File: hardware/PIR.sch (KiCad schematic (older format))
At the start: 3 parts, among them U10 EKMC1601112

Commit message: update
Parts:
- R18, R20: footprint Resistors_SMD:R_0603_HandSoldering -> Resistor_SMD:R_0603_1608Metric_Pad1.05x0.95mm_HandSolder
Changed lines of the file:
@@
 F 0 "R18" V 6050 2275 50  0000 C CNN
 F 1 "R_100k" V 5950 2275 50  0000 C CNN
-F 2 "Resistors_SMD:R_0603_HandSoldering" V 5980 2275 50  0001 C CNN
+F 2 "Resistor_SMD:R_0603_1608Metric_Pad1.05x0.95mm_HandSolder" V 5980 2275 50  0001 C CNN
 F 3 "https://www.digikey.com/product-detail/en/yageo/RC0603JR-07100KL/311-100KGRCT-ND/729645" V 6130 2275 50  0001 C CNN
 F 4 "RC0603JR-07100KL" V 6230 2375 60  0001 C CNN "Part Number"
@@
 F 0 "R20" V 6275 2475 50  0000 C CNN
 F 1 "R_100k" V 6175 2475 50  0000 C CNN
-F 2 "Resistors_SMD:R_0603_HandSoldering" V 6205 2475 50  0001 C CNN
+F 2 "Resistor_SMD:R_0603_1608Metric_Pad1.05x0.95mm_HandSolder" V 6205 2475 50  0001 C CNN
 F 3 "https://www.digikey.com/product-detail/en/yageo/RC0603JR-07100KL/311-100KGRCT-ND/729645" V 6355 2475 50  0001 C CNN
 F 4 "RC0603JR-07100KL" V 6455 2575 60  0001 C CNN "Part Number"

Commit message: order complete
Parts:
- R18, R20: Part Number RC0603JR-07100KL -> ERA-3AEB104V
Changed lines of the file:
@@
 F 2 "Resistor_SMD:R_0603_1608Metric_Pad1.05x0.95mm_HandSolder" V 5980 2275 50  0001 C CNN
 F 3 "https://www.digikey.com/product-detail/en/yageo/RC0603JR-07100KL/311-100KGRCT-ND/729645" V 6130 2275 50  0001 C CNN
-F 4 "RC0603JR-07100KL" V 6230 2375 60  0001 C CNN "Part Number"
+F 4 "ERA-3AEB104V" V 6230 2375 60  0001 C CNN "Part Number"
 	1    6050 2275
 	0    1    1    0
@@
 F 2 "Resistor_SMD:R_0603_1608Metric_Pad1.05x0.95mm_HandSolder" V 6205 2475 50  0001 C CNN
 F 3 "https://www.digikey.com/product-detail/en/yageo/RC0603JR-07100KL/311-100KGRCT-ND/729645" V 6355 2475 50  0001 C CNN
-F 4 "RC0603JR-07100KL" V 6455 2575 60  0001 C CNN "Part Number"
+F 4 "ERA-3AEB104V" V 6455 2575 60  0001 C CNN "Part Number"
 	1    6275 2475
 	-1   0    0    1

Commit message: update schematic
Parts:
- removed R18: R_100k, Resistor_SMD:R_0603_1608Metric_Pad1.05x0.95mm_HandSolder, symbol liger-rescue:R_100k
- removed U10: EKMC1601112, open-automation:EKMC1601112, symbol liger-rescue:EKMC1601112
- added C3: C_0.1uF, Capacitor_SMD:C_0603_1608Metric_Pad1.05x0.95mm_HandSolder, symbol open-automation:C_0.1uF
- added C4: C_100pF, Capacitor_SMD:C_0603_1608Metric_Pad1.05x0.95mm_HandSolder, symbol open-automation:C_100pF
- added R8: R_47.5, Resistor_SMD:R_0603_1608Metric_Pad1.05x0.95mm_HandSolder, symbol open-automation:R_47.5
- added U7: PYQ2898, open-automation:PYQ2898, symbol open-automation:PYQ2898
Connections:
- wire segments 8 -> 15
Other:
- moved on the sheet: R20
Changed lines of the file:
@@
 L power:GND #PWR029
 U 1 1 59B7E3DB
-P 5125 2375
-F 0 "#PWR029" H 5125 2125 50  0001 C CNN
-F 1 "GND" H 5125 2225 50  0000 C CNN
-F 2 "" H 5125 2375 50  0000 C CNN
-F 3 "" H 5125 2375 50  0000 C CNN
-	1    5125 2375
+P 5100 3250
+F 0 "#PWR029" H 5100 3000 50  0001 C CNN
+F 1 "GND" H 5100 3100 50  0000 C CNN
+F 2 "" H 5100 3250 50  0000 C CNN
+F 3 "" H 5100 3250 50  0000 C CNN
+	1    5100 3250
 	1    0    0    -1
-$EndComp
-$Comp
-L liger-rescue:R_100k R18
-U 1 1 5A160B80
-P 6050 2275
-F 0 "R18" V 6050 2275 50  0000 C CNN
-F 1 "R_100k" V 5950 2275 50  0000 C CNN
-F 2 "Resistor_SMD:R_0603_1608Metric_Pad1.05x0.95mm_HandSolder" V 5980 2275 50  0001 C CNN
-F 3 "https://www.digikey.com/product-detail/en/yageo/RC0603JR-07100KL/311-100KGRCT-ND/729645" V 6130 2275 50  0001 C CNN
-F 4 "ERA-3AEB104V" V 6230 2375 60  0001 C CNN "Part Number"
-	1    6050 2275
-	0    1    1    0
 $EndComp
 $Comp
 L liger-rescue:R_100k R20
 U 1 1 5A1610DC
-P 6275 2475
-F 0 "R20" V 6275 2475 50  0000 C CNN
-F 1 "R_100k" V 6175 2475 50  0000 C CNN
-F 2 "Resistor_SMD:R_0603_1608Metric_Pad1.05x0.95mm_HandSolder" V 6205 2475 50  0001 C CNN
-F 3 "https://www.digikey.com/product-detail/en/yageo/RC0603JR-07100KL/311-100KGRCT-ND/729645" V 6355 2475 50  0001 C CNN
-F 4 "ERA-3AEB104V" V 6455 2575 60  0001 C CNN "Part Number"
-	1    6275 2475
+P 6450 3150
+F 0 "R20" V 6450 3150 50  0000 C CNN
+F 1 "R_100k" V 6350 3150 50  0000 C CNN
+F 2 "Resistor_SMD:R_0603_1608Metric_Pad1.05x0.95mm_HandSolder" V 6380 3150 50  0001 C CNN
+F 3 "https://www.digikey.com/product-detail/en/yageo/RC0603JR-07100KL/311-100KGRCT-ND/729645" V 6530 3150 50  0001 C CNN
+F 4 "ERA-3AEB104V" V 6630 3250 60  0001 C CNN "Part Number"
+	1    6450 3150
 	-1   0    0    1
 $EndComp
-Wire Wire Line
-	5125 2375 5125 2350
-Wire Wire Line
-	5125 2350 5175 2350
-Wire Wire Line
-	5050 2200 5175 2200
-Wire Wire Line
-	5900 2275 5775 2275
-Wire Wire Line
-	6200 2275 6275 2275
-Wire Wire Line
-	6275 2275 6275 2325
 $Comp
 L power:GND #PWR030
 U 1 1 5A1624EE
-P 6275 2675
-F 0 "#PWR030" H 6275 2425 50  0001 C CNN
-F 1 "GND" H 6275 2525 50  0000 C CNN
-F 2 "" H 6275 2675 50  0000 C CNN
-F 3 "" H 6275 2675 50  0000 C CNN
-	1    6275 2675
+P 6450 3350
+F 0 "#PWR030" H 6450 3100 50  0001 C CNN
+F 1 "GND" H 6450 3200 50  0000 C CNN
+F 2 "" H 6450 3350 50  0000 C CNN
+F 3 "" H 6450 3350 50  0000 C CNN
+	1    6450 3350
+	1    0    0    -1
+$EndComp
+Text HLabel 4850 2850 0    60   Input ~ 0
+3V3
+Text HLabel 6600 2950 2    60   Input ~ 0
+PIR
+$Comp
+L open-automation:PYQ2898 U7
+U 1 1 5BA828EE
+P 5450 2950
+F 0 "U7" H 5650 2750 60  0000 C CNN
+F 1 "PYQ2898" H 5500 3191 60  0000 C CNN
+F 2 "open-automation:PYQ2898" H 5500 2550 60  0001 C CNN
+F 3 "https://datasheet.octopart.com/PYQ2898-Excelitas-Technology-datasheet-9789873.pdf" H 5600 2650 60  0001 C CNN
+F 4 "PYQ2898" H 5450 3250 60  0001 C CNN "Part Number"
+	1    5450 2950
 	1    0    0    -1
 $EndComp
 Wire Wire Line
-	6275 2675 6275 2625
-Connection ~ 6275 2275
+	6300 2950 6450 2950
+Wire Wire Line
+	6450 3000 6450 2950
+Connection ~ 6450 2950
+Wire Wire Line
+	6450 2950 6600 2950
+Wire Wire Line
+	6450 3350 6450 3300
 $Comp
-L liger-rescue:EKMC1601112 U10
-U 1 1 5A1702E3
-P 5425 2275
-F 0 "U10" H 5625 2100 60  0000 C CNN
-F 1 "EKMC1601112" H 5425 2475 60  0000 C CNN
-F 2 "open-automation:EKMC1601112" H 5575 1950 60  0001 C CNN
-F 3 "https://www.digikey.com/products/en?keywords=EKMC1601112" H 5575 2025 60  0001 C CNN
-F 4 "EKMC1601112" H 5425 2575 60  0001 C CNN "Part Number"
-	1    5425 2275
+L open-automation:C_0.1uF C3
+U 1 1 5BA837C7
+P 5000 3050
+F 0 "C3" H 4900 3150 50  0000 L CNN
+F 1 "C_0.1uF" H 4700 2950 50  0000 L CNN
+F 2 "Capacitor_SMD:C_0603_1608Metric_Pad1.05x0.95mm_HandSolder" H 5100 3350 50  0001 C CNN
+F 3 "https://www.digikey.com/product-detail/en/tdk-corporation/C1608X8R1H104K080AB/445-8818-1-ND/3248223" H 5000 2800 50  0001 C CNN
+F 4 "CL10F104ZO8NNNC" H 5125 3250 60  0001 C CNN "Part Number"
+	1    5000 3050
 	1    0    0    -1
 $EndComp
 Wire Wire Line
-	6275 2275 6425 2275
-Text HLabel 5050 2200 0    60   Input ~ 0
-3V3
-Text HLabel 6425 2275 2    60   Input ~ 0
-PIR
+	4850 2850 5000 2850
+Wire Wire Line
+	5000 2900 5000 2850
+Connection ~ 5000 2850
+Wire Wire Line
+	5000 2850 5200 2850
+Wire Wire Line
+	5000 3200 5100 3200
+Wire Wire Line
+	5200 3200 5200 3050
+Wire Wire Line
+	5100 3250 5100 3200
+Connection ~ 5100 3200
+Wire Wire Line
+	5100 3200 5200 3200
+$Comp
+L open-automation:C_100pF C4
+U 1 1 5BA83E1B
+P 5900 3200
+F 0 "C4" H 5950 3300 50  0000 L CNN
+F 1 "C_100pF" H 5950 3100 50  0000 L CNN
+F 2 "Capacitor_SMD:C_0603_1608Metric_Pad1.05x0.95mm_HandSolder" H 6000 3500 50  0001 C CNN
+F 3 "https://www.digikey.com/product-detail/en/avx-corporation/06035A101FAT2A/478-6202-1-ND/2391401" H 5900 2950 50  0001 C CNN
+F 4 "06035A101FAT2A" H 6025 3400 60  0001 C CNN "Part Number"
+	1    5900 3200
+	1    0    0    -1
+$EndComp
+$Comp
+L open-automation:R_47.5 R8
+U 1 1 5BA85345
+P 6150 2950
+F 0 "R8" V 6150 2950 50  0000 C CNN
+F 1 "R_47.5" V 6050 2950 50  0000 C CNN
+F 2 "Resistor_SMD:R_0603_1608Metric_Pad1.05x0.95mm_HandSolder" V 6080 2950 50  0001 C CNN
+F 3 "https://www.digikey.com/product-detail/en/yageo/RC0603FR-0747R5L/311-47.5HRCT-ND/730201" V 6230 2950 50  0001 C CNN
+F 4 "ERJ-3EKF47R5V" V 6330 3050 60  0001 C CNN "Part Number"
+	1    6150 2950
+	0    1    1    0
+$EndComp
+Wire Wire Line
+	5800 2950 5900 2950
+Wire Wire Line
+	5900 3050 5900 2950
+Connection ~ 5900 2950
+Wire Wire Line
+	5900 2950 6000 2950
+$Comp
+L power:GND #PWR0103
+U 1 1 5BA8569A
+P 5900 3400
+F 0 "#PWR0103" H 5900 3150 50  0001 C CNN
+F 1 "GND" H 5900 3250 50  0000 C CNN
+F 2 "" H 5900 3400 50  0000 C CNN
+F 3 "" H 5900 3400 50  0000 C CNN
+	1    5900 3400
+	1    0    0    -1
+$EndComp
+Wire Wire Line
+	5900 3350 5900 3400
 $EndSCHEMATC

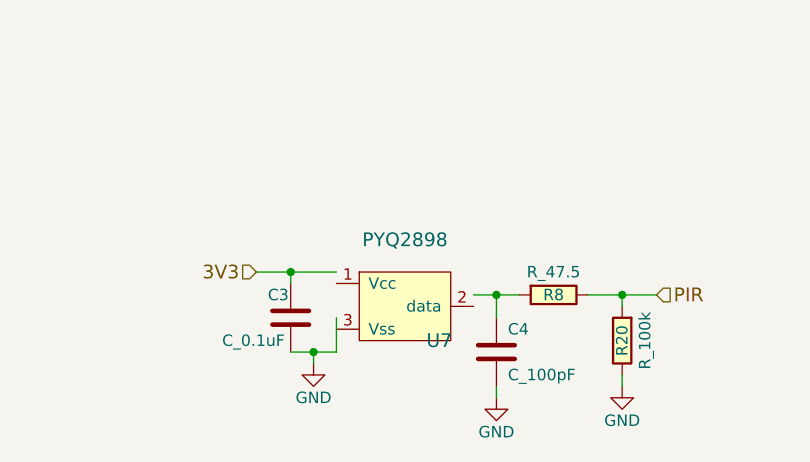
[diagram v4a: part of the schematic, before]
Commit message: update button
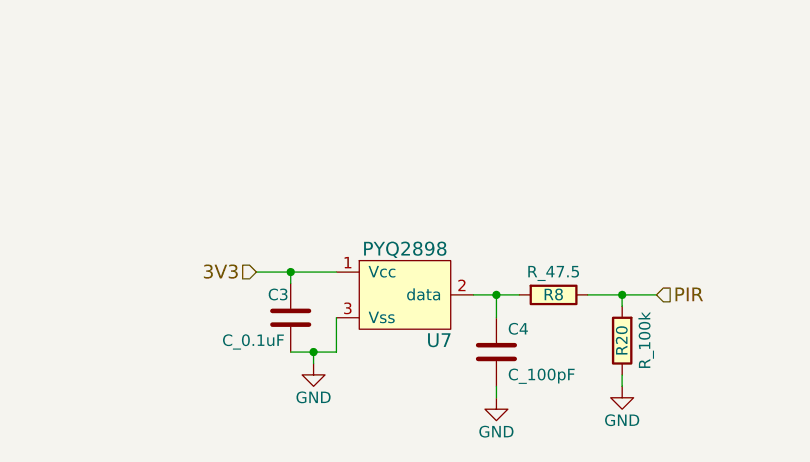
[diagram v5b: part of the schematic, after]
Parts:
- U7: footprint open-automation:PYQ2898 -> Package_TO_SOT_THT:TO-5-3
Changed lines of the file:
@@
 Text HLabel 6600 2950 2    60   Input ~ 0
 PIR
-$Comp
-L open-automation:PYQ2898 U7
-U 1 1 5BA828EE
-P 5450 2950
-F 0 "U7" H 5650 2750 60  0000 C CNN
-F 1 "PYQ2898" H 5500 3191 60  0000 C CNN
-F 2 "open-automation:PYQ2898" H 5500 2550 60  0001 C CNN
-F 3 "https://datasheet.octopart.com/PYQ2898-Excelitas-Technology-datasheet-9789873.pdf" H 5600 2650 60  0001 C CNN
-F 4 "PYQ2898" H 5450 3250 60  0001 C CNN "Part Number"
-	1    5450 2950
-	1    0    0    -1
-$EndComp
 Wire Wire Line
 	6300 2950 6450 2950
@@
 Wire Wire Line
 	5000 3200 5100 3200
-Wire Wire Line
-	5200 3200 5200 3050
 Wire Wire Line
 	5100 3250 5100 3200
@@
 Wire Wire Line
 	5900 3350 5900 3400
+Wire Wire Line
+	5200 3200 5200 3050
+$Comp
+L open-automation:PYQ2898 U7
+U 1 1 5BB8B302
+P 5450 2900
+F 0 "U7" H 5650 2650 60  0000 C CNN
+F 1 "PYQ2898" H 5500 3050 60  0000 C CNN
+F 2 "Package_TO_SOT_THT:TO-5-3" H 5450 2900 60  0001 C CNN
+F 3 "" H 5450 2900 60  0001 C CNN
+F 4 "PYQ2898" H 5450 2900 50  0001 C CNN "Part Number"
+	1    5450 2900
+	1    0    0    -1
+$EndComp
 $EndSCHEMATC
